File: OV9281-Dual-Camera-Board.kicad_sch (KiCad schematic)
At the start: 82 parts, among them J3 Conn_FFC_WE_68715014522_TWO-S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, Q1 BSS138AKA, U1 ImageSensor_OV9281, U2 ImageSensor_OV9281, U3 NTS0104BQ, U4 NTB0104BQ, U5 TLV73318PDBVT, U6 TLV73312PDBVT, U7 TLV73328PDBVT, Y1 7C-24.000MBB-T, Y2 7C-24.000MBB-T

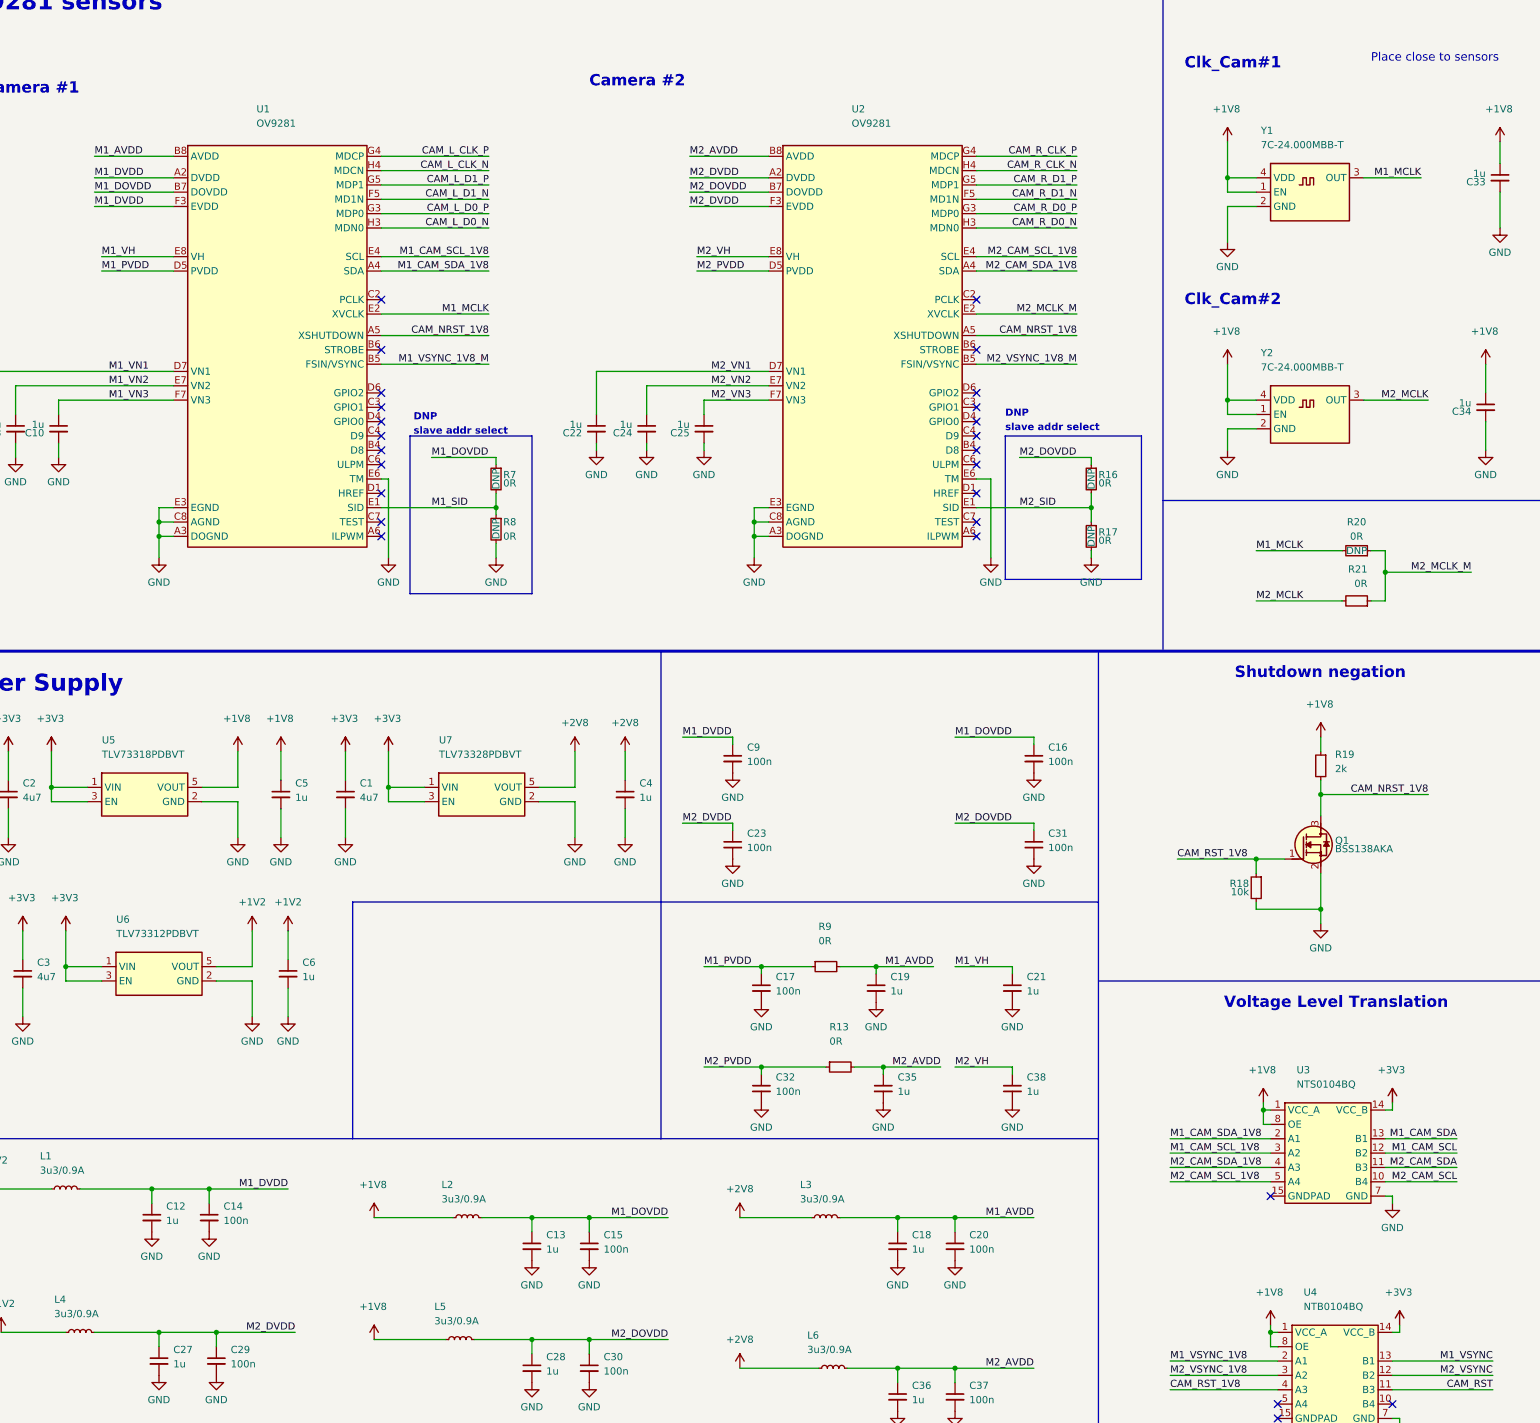
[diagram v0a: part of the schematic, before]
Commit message: Update components from library
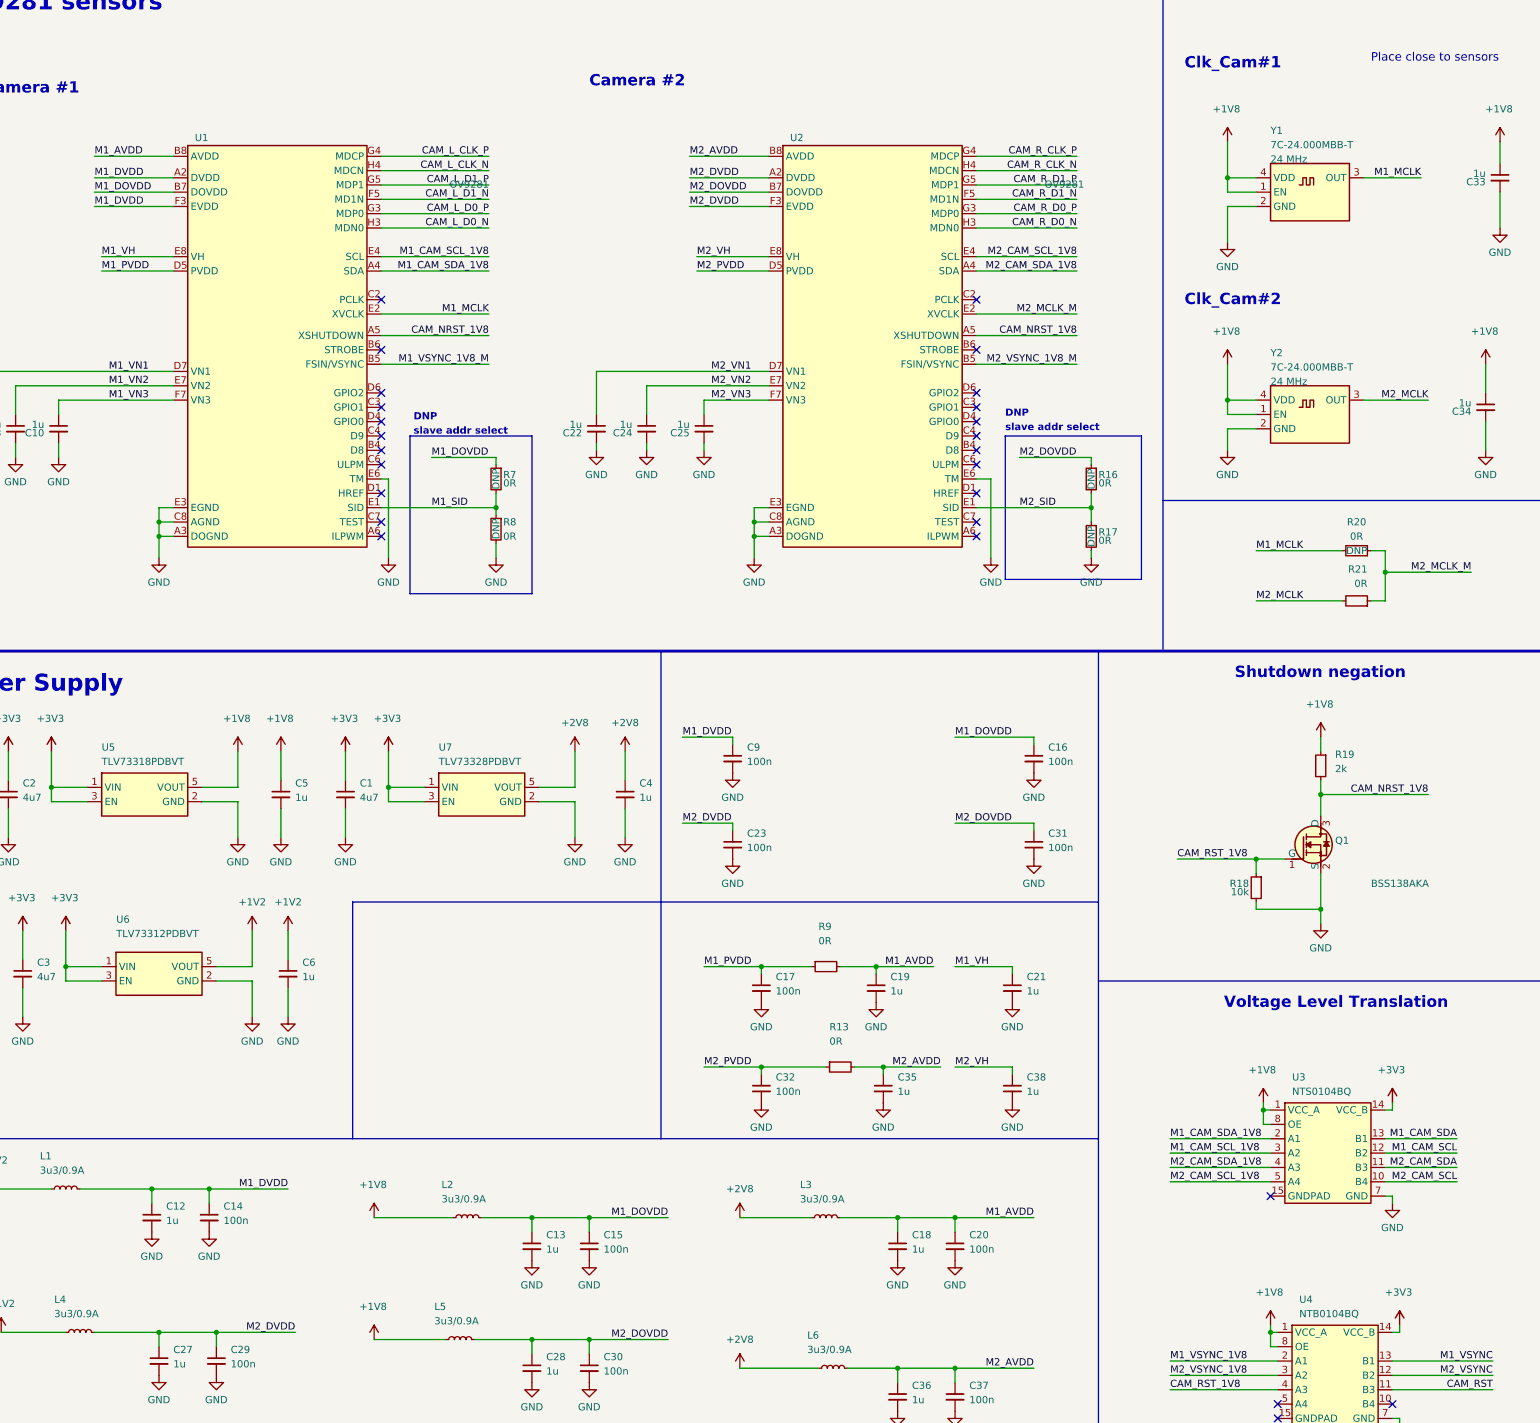
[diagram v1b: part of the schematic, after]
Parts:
- U1, U2: footprint antmicro-footprints:ImageSensor_OV9281 -> antmicro-footprints:OV9281; symbol antmicroCameramodules:ImageSensor_OV9281 -> antmicroCameramodules:OV9281; Manufacturer ARDUCAM -> OmniVision
- Y1, Y2: footprint antmicro-footprints:7C-24.000MBB-T -> antmicro-footprints:Oscillator_SMD_TXC_7C_5x3.2x1.2mm; symbol antmicroOscillators:7C-24.000MBB-T -> antmicroOscillators:Oscillator_24MHz_TXC_7C; Val (none) -> 24 MHz
